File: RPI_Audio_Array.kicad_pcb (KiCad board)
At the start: 2 copper layers, 66.9 x 99.9 mm, 75 parts, among them J1 Conn_02x20_Odd_Even, U1 PCMD3140IRTER, U2 SPH0690LM4H-1, U3 SPH0690LM4H-1, U4 SPH0690LM4H-1, U5 SPH0690LM4H-1, U6 TLV7103318QDSERQ1

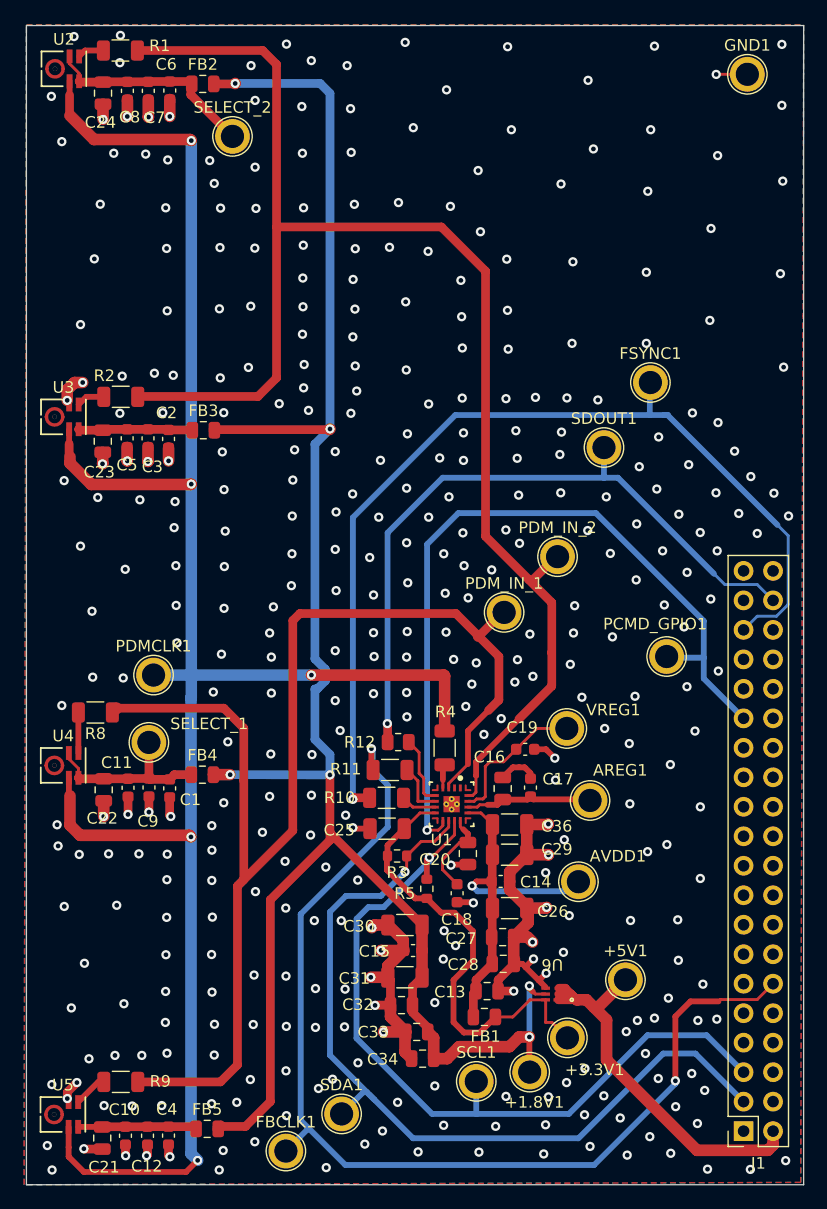
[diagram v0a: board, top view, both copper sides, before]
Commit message: updated PCB and schematic for review
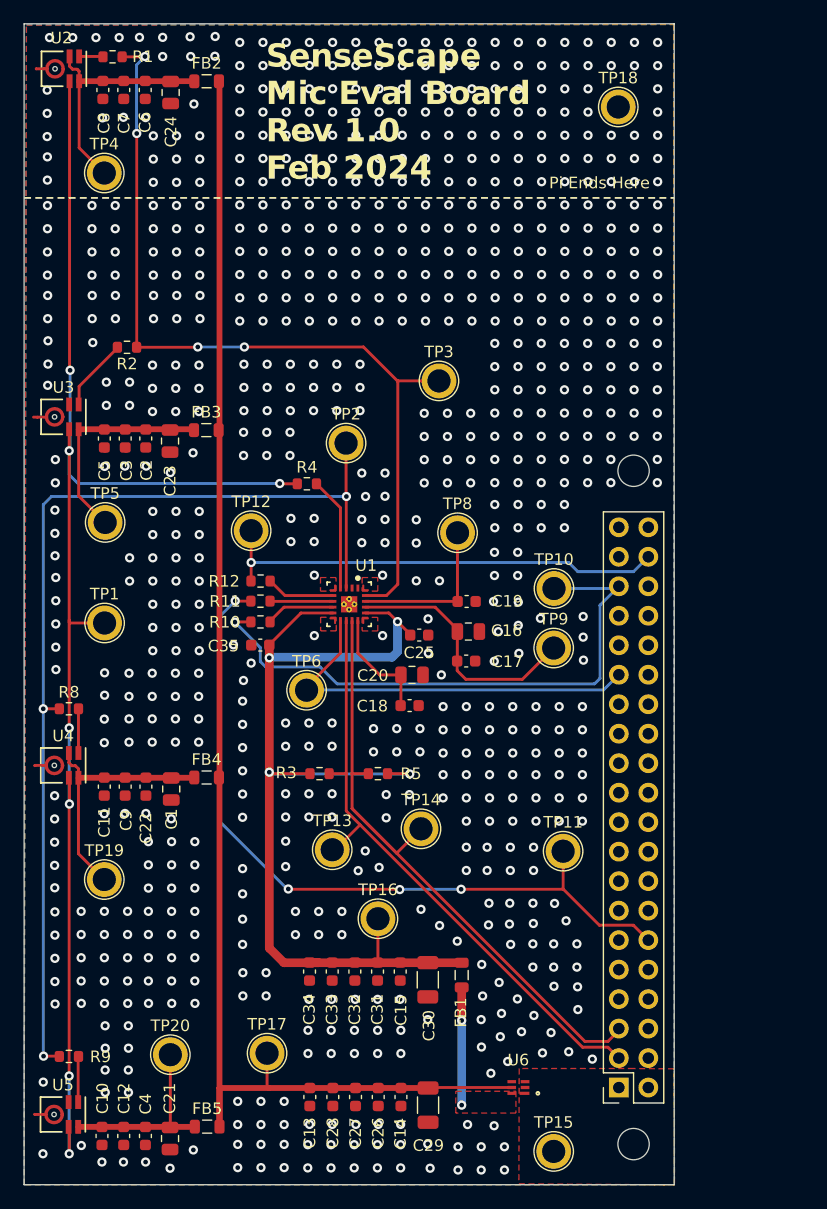
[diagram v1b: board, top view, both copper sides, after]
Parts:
- removed +1.8V1, +3.3V1, +5V1, AREG1, AVDD1, FBCLK1, FSYNC1, GND1, PCMD_GPIO1, PDMCLK1, PDM_IN_1, PDM_IN_2, SCL1, SDA1, SDOUT1, SELECT_1, SELECT_2, VREG1: TestPoint, TestPoint:TestPoint_Plated_Hole_D2.0mm
- removed C36: 100nf, Capacitor_SMD:C_1206_3216Metric
- added C35: 100nF, Capacitor_SMD:C_0603_1608Metric, F.Cu at (48.8, 79.4)
- added H1: MountingHole, MountingHole:MountingHole_2.7mm_M2.5, F.Cu at (81.0, 122.4)
- added H2: MountingHole, MountingHole:MountingHole_2.7mm_M2.5, F.Cu at (81.0, 64.4)
- added TP1: PDMCLK, TestPoint:TestPoint_Plated_Hole_D2.0mm, F.Cu at (35.4, 77.5)
- added TP10: FSYNC, TestPoint:TestPoint_Plated_Hole_D2.0mm, F.Cu at (74.1, 74.5)
- added TP11: FBCLK, TestPoint:TestPoint_Plated_Hole_D2.0mm, F.Cu at (74.9, 97.2)
- added TP12: SDOUT, TestPoint:TestPoint_Plated_Hole_D2.0mm, F.Cu at (48.0, 69.6)
- added TP13: SDA, TestPoint:TestPoint_Plated_Hole_D2.0mm, F.Cu at (55.0, 97.0)
- added TP14: SCL, TestPoint:TestPoint_Plated_Hole_D2.0mm, F.Cu at (62.6, 95.2)
- added TP15: 5V, TestPoint:TestPoint_Plated_Hole_D2.0mm, F.Cu at (74.1, 123.0)
- added TP16: 3V3, TestPoint:TestPoint_Plated_Hole_D2.0mm, F.Cu at (58.9, 103.0)
- added TP17: 1V8, TestPoint:TestPoint_Plated_Hole_D2.0mm, F.Cu at (49.4, 114.6)
- added TP18: GND, TestPoint:TestPoint_Plated_Hole_D2.0mm, F.Cu at (79.6, 33.1)
- added TP19: PDMVDD3, TestPoint:TestPoint_Plated_Hole_D2.0mm, F.Cu at (35.4, 99.6)
- added TP2: PDMIN1, TestPoint:TestPoint_Plated_Hole_D2.0mm, F.Cu at (56.2, 62.0)
- added TP20: PDMVDD4, TestPoint:TestPoint_Plated_Hole_D2.0mm, F.Cu at (41.0, 114.7)
- added TP3: PDMIN2, TestPoint:TestPoint_Plated_Hole_D2.0mm, F.Cu at (64.2, 56.7)
- added TP4: PDMVDD2, TestPoint:TestPoint_Plated_Hole_D2.0mm, F.Cu at (35.4, 38.8)
- added TP5: PDMVDD2, TestPoint:TestPoint_Plated_Hole_D2.0mm, F.Cu at (35.4, 68.9)
- added TP6: PCM_IO1, TestPoint:TestPoint_Plated_Hole_D2.0mm, F.Cu at (52.8, 83.3)
- added TP8: VREF, TestPoint:TestPoint_Plated_Hole_D2.0mm, F.Cu at (65.8, 69.7)
- added TP9: AREG, TestPoint:TestPoint_Plated_Hole_D2.0mm, F.Cu at (74.1, 79.7)
- C1, C17, C18, C19, C2, C4, C6: value 0.1uf -> 100nF
- C10, C3, C7, C9: value 47pf -> 47pF
- C11, C12, C5, C8: value 330pf -> 330pF
- C13, C32: value 10nf -> 10nF; footprint Capacitor_SMD:C_0805_2012Metric -> Capacitor_SMD:C_0603_1608Metric
- C14, C15: value 1uf -> 1uF
- C16, C20, C29, C30: value 10uf -> 10uF
- C21, C22, C23, C24: value 2.2uf -> 2.2uF
- C25, C26, C31: value 100nf -> 100nF; footprint Capacitor_SMD:C_1206_3216Metric -> Capacitor_SMD:C_0603_1608Metric
- C27, C33: value 1nf -> 1nF; footprint Capacitor_SMD:C_0805_2012Metric -> Capacitor_SMD:C_0603_1608Metric
- C28, C34: value 100pf -> 100pF; footprint Capacitor_SMD:C_0805_2012Metric -> Capacitor_SMD:C_0603_1608Metric
- FB1, FB2, FB3, FB4, FB5: footprint Capacitor_SMD:C_0805_2012Metric -> Inductor_SMD:L_0805_2012Metric
- R1, R2, R4, R8, R9: value 100 -> 100Ω; footprint Resistor_SMD:R_1206_3216Metric -> Resistor_SMD:R_0603_1608Metric
- R10, R11: value 0 -> 0Ω; footprint Resistor_SMD:R_1206_3216Metric -> Resistor_SMD:R_0603_1608Metric
- R12: value 33 -> 33Ω; footprint Resistor_SMD:R_0805_2012Metric -> Resistor_SMD:R_0603_1608Metric
- R3, R5: value 4K7 -> 4K7Ω
- moved J1 29.5 mm to (81.0, 93.4)
- moved R4 25.7 mm to (52.8, 65.5), turned to 0 degrees
- moved C29 22.7 mm to (63.2, 119.0), turned to -90 degrees
- moved C14 20.5 mm to (60.9, 118.3), turned to -90 degrees
- moved C26 19.8 mm to (59.0, 118.3), turned to -90 degrees
- moved U1 19.4 mm to (56.5, 75.9)
- moved C27 18.7 mm to (57.0, 118.3), turned to -90 degrees
- moved R10 18.6 mm to (48.8, 77.4)
- moved C28 18.6 mm to (55.0, 118.3), turned to -90 degrees
- moved R11 18.3 mm to (48.8, 75.6)
- moved R12 18.2 mm to (48.8, 73.9)
- moved C13 17.8 mm to (53.1, 118.3), turned to -90 degrees
- moved C25 16.9 mm to (62.5, 78.6), turned to 0 degrees
- moved C18 16.7 mm to (61.7, 84.6), turned to 0 degrees
- moved C20 16.1 mm to (61.9, 82.0), turned to 0 degrees
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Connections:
- net Net-(U3-VDD) renamed PDM_VDD2
- net Net-(U5-VDD) renamed PDM_VDD4
- net SELECT_1 renamed PDM_VDD3
- net SELECT_2 renamed PDM_VDD1
- C13 pad 1: AVDD -> +1V8
- C14 pad 1: AVDD -> +1V8
- C15 pad 1: FILTER_BANK_1 -> +3V3
- C25 pad 1: IOVDD -> +3V3
- C26 pad 1: AVDD -> +1V8
- C27 pad 1: AVDD -> +1V8
- C28 pad 1: AVDD -> +1V8
- C29 pad 1: AVDD -> +1V8
- C30 pad 1: FILTER_BANK_1 -> +3V3
- C31 pad 1: FILTER_BANK_1 -> +3V3
- C32 pad 1: FILTER_BANK_1 -> +3V3
- C33 pad 1: FILTER_BANK_1 -> +3V3
- C34 pad 1: FILTER_BANK_1 -> +3V3
- FB1 pad 1: IOVDD -> Net-(U6-OUT1)
- FB1 pad 2: AVDD -> +3V3
- FB2 pad 2: FILTER_BANK_1 -> +1V8
- FB3 pad 2: FILTER_BANK_1 -> +1V8
- FB4 pad 2: FILTER_BANK_1 -> +1V8
- FB5 pad 2: FILTER_BANK_1 -> +1V8
- J1 pad 14: unconnected-(J1-Pin_14-Pad14) -> GND
- J1 pad 20: unconnected-(J1-Pin_20-Pad20) -> GND
- J1 pad 25: unconnected-(J1-Pin_25-Pad25) -> GND
- J1 pad 30: unconnected-(J1-Pin_30-Pad30) -> GND
- J1 pad 34: unconnected-(J1-Pin_34-Pad34) -> GND
- J1 pad 39: unconnected-(J1-Pin_39-Pad39) -> GND
- J1 pad 6: unconnected-(J1-Pin_6-Pad6) -> GND
- J1 pad 9: unconnected-(J1-Pin_9-Pad9) -> GND
- R3 pad 2: IOVDD -> +3V3
- R5 pad 2: IOVDD -> +3V3
- U1 pad 16: AVDD -> +3V3
- U1 pad 9: IOVDD -> +3V3
- U1 pad V: (no net) -> GND
- U6 pad 5: FILTER_BANK_1 -> +1V8
- U6 pad 6: IOVDD -> Net-(U6-OUT1)
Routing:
- net FILTER_BANK_1: track 169.1 -> 0.00 mm, vias 6 -> 0
- net +1V8: track 0.00 -> 120.7 mm
- net +3V3: track 0.00 -> 90.2 mm, vias 0 -> 4
- net GND: track 91.8 -> 4.22 mm, vias 382 -> 775
- net PDMCLK: track 176.0 -> 124.1 mm, vias 5 -> 7
- net PDM_IN_2: track 125.4 -> 75.3 mm, vias 0 -> 4
- net IOVDD: track 39.4 -> 0.00 mm
- net PCMD_GPIO1: track 68.4 -> 32.5 mm, vias 1 -> 0
- net FSYNC: track 85.0 -> 49.9 mm
- net +5V: track 34.6 -> 0.00 mm
- net AVDD: track 31.3 -> 0.00 mm, vias 1 -> 0
- net FBCLK: track 92.6 -> 65.4 mm, vias 2 -> 4
- net PDM_IN_1: track 111.2 -> 89.1 mm, vias 0 -> 3
- net SDOUT: track 60.3 -> 39.4 mm
- net SDA: track 73.8 -> 53.2 mm, vias 1 -> 0
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- added copper zone on F.Cu, net +5V
- added copper zone on F.Cu, net Net-(U6-OUT1)
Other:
- board size 66.9 x 99.9 mm -> 56 x 100 mm
- board text added: "Pi Ends Here"
- board text added: "SenseScape Mic Eval Board Rev 1.0 Feb 2024"
